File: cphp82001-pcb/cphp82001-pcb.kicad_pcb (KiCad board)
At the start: 2 copper layers, 56 x 44 mm, 32 parts, among them J1 USB_B_Micro, J2 PAD+, J3 PAD-, Q1 2N7002, U1 BQ21040, U2 TLV75801, U3 MAX40203AUK, U6 NCP360SNT

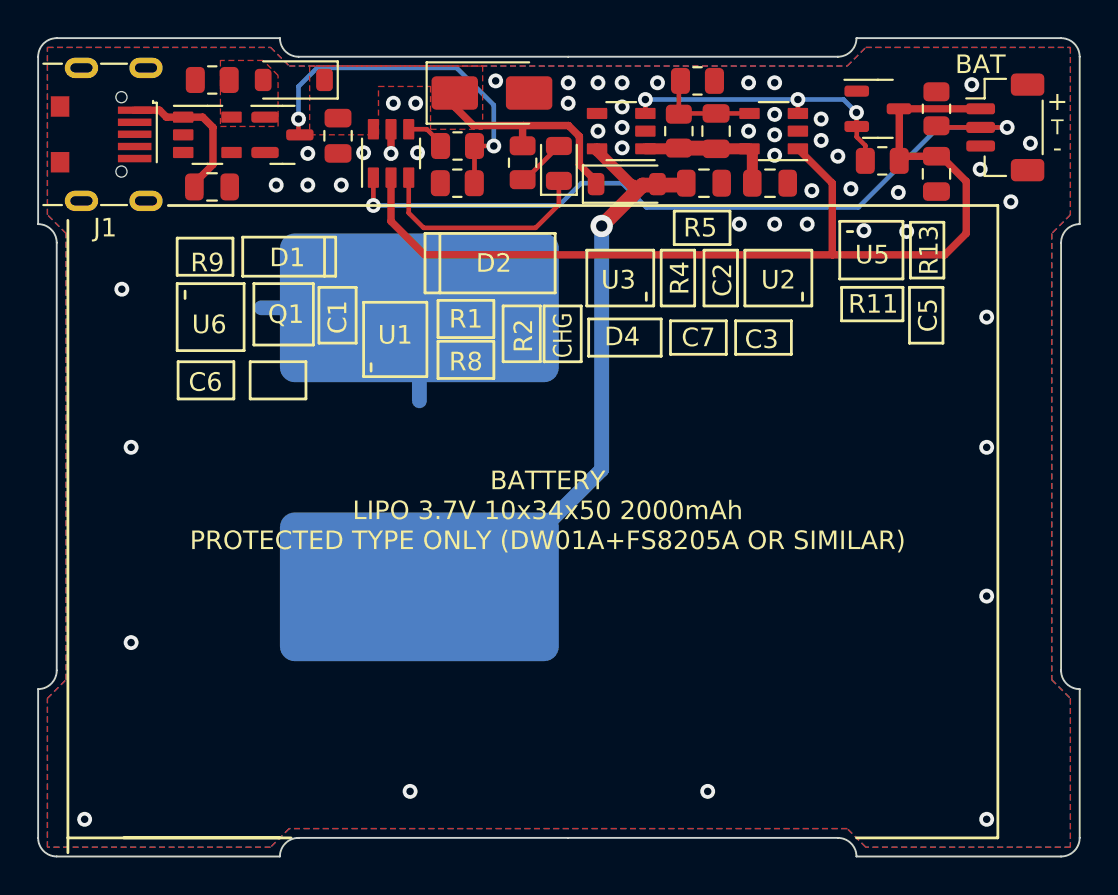
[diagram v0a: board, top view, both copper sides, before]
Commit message: rev3.3
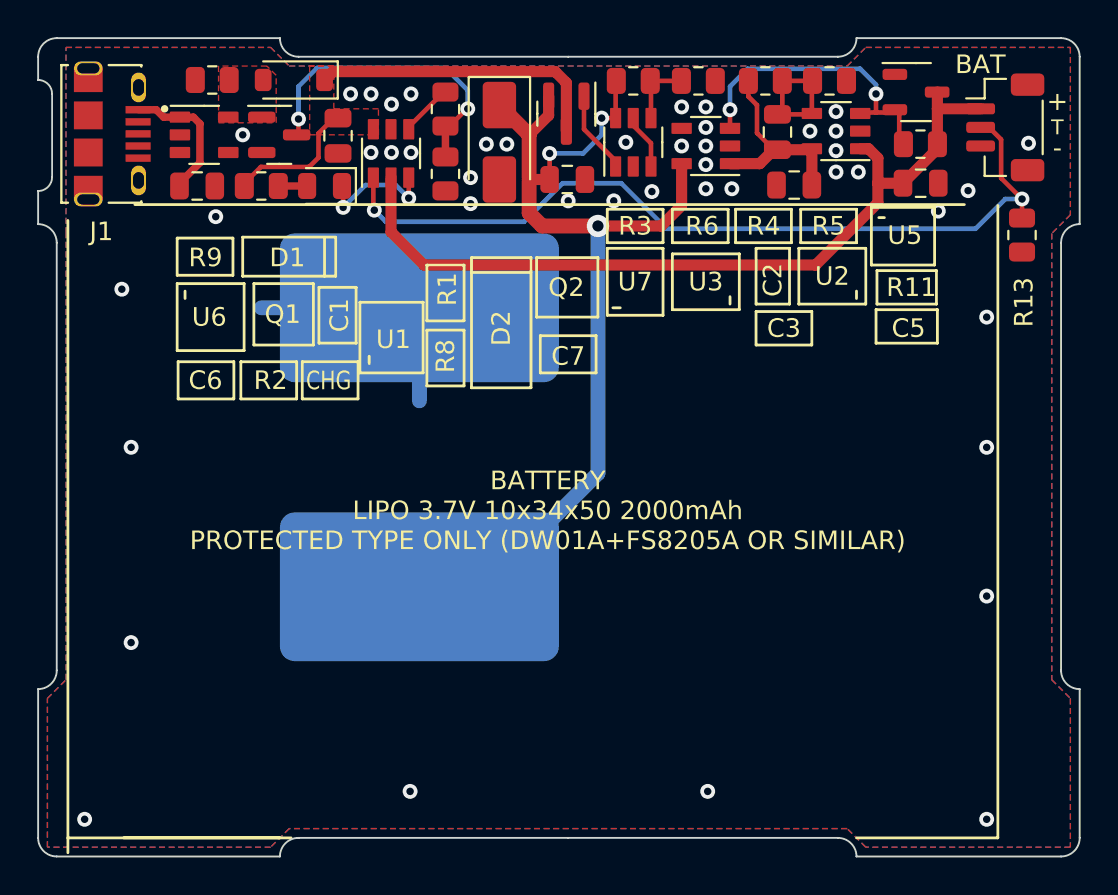
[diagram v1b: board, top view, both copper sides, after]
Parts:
- removed D4: PMEG40T10ERX, Diode_SMD:D_SOD-123
- added Q2: AO3401A, Package_TO_SOT_SMD:SOT-23, F.Cu at (28.4, 4.06)
- added R3: 560k, Resistor_SMD:R_0805_2012Metric, F.Cu at (32.0, 2.30)
- added R6: 220k, Resistor_SMD:R_0805_2012Metric, F.Cu at (35.5, 2.30)
- added U7: MCP65R41T-120E/CHY, george:SOT-23-6_TI_DBV6, F.Cu at (32.0, 5.60)
- J1: value USB_B_Micro -> USB; footprint george:USB_ALIEX_4LEG -> mod_local:AMPHENOL_10118194-0001LF
- U5: value ~ -> APX803S-SA
- moved R2 14.1 mm to (12.0, 7.95), turned to 180 degrees
- moved D3 12.7 mm to (15.4, 7.95), turned to 180 degrees
- moved R13 8.20 mm to (52.9, 10.6), turned to 90 degrees
- moved C7 7.35 mm to (28.4, 7.60)
- moved R5 7.10 mm to (42.5, 2.30)
- moved R4 5.38 mm to (39.1, 2.30), turned to 0 degrees
- moved U3 4.62 mm to (35.9, 5.80)
- moved U2 3.35 mm to (42.9, 5.00)
- moved C2 3.30 mm to (39.8, 5.05)
- moved D2 2.68 mm to (24.8, 5.60), turned to -90 degrees
- moved J1 2.52 mm to (2.70, 5.15)
- moved U5 2.24 mm to (47.2, 2.90)
- moved R11 2.24 mm to (47.4, 5.70)
- moved R1 2.09 mm to (21.9, 3.81), turned to 90 degrees
- moved C3 1.30 mm to (40.6, 7.90), turned to 180 degrees
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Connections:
- D2 pad 1: /VCC -> /VOUT
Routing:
- net /VOUT: track 30.7 -> 51.3 mm, vias 1 -> 3
- net /VCC: track 12.0 -> 23.1 mm
- net /B+: track 54.6 -> 43.9 mm
- net /CHG: track 11.9 -> 6.50 mm, vias 0 -> 2
- net /PASSG: track 0.00 -> 4.48 mm
- net /VCOMP: track 0.00 -> 3.64 mm
- net /VREG: track 7.44 -> 10.7 mm
- net /TS: track 41.9 -> 45.0 mm
- net /PROG2: track 19.6 -> 16.9 mm
- net Net-(U7-+): track 0.00 -> 2.59 mm
- net /ADJ: track 5.46 -> 6.78 mm
- net /GND: track 14.5 -> 13.5 mm, vias 50 -> 44
- net /LCHG: track 2.56 -> 1.55 mm
- net /PROG: track 2.02 -> 2.75 mm
- net /VBUS1: track 8.01 -> 7.29 mm
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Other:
- outline, holes or cut-outs redrawn

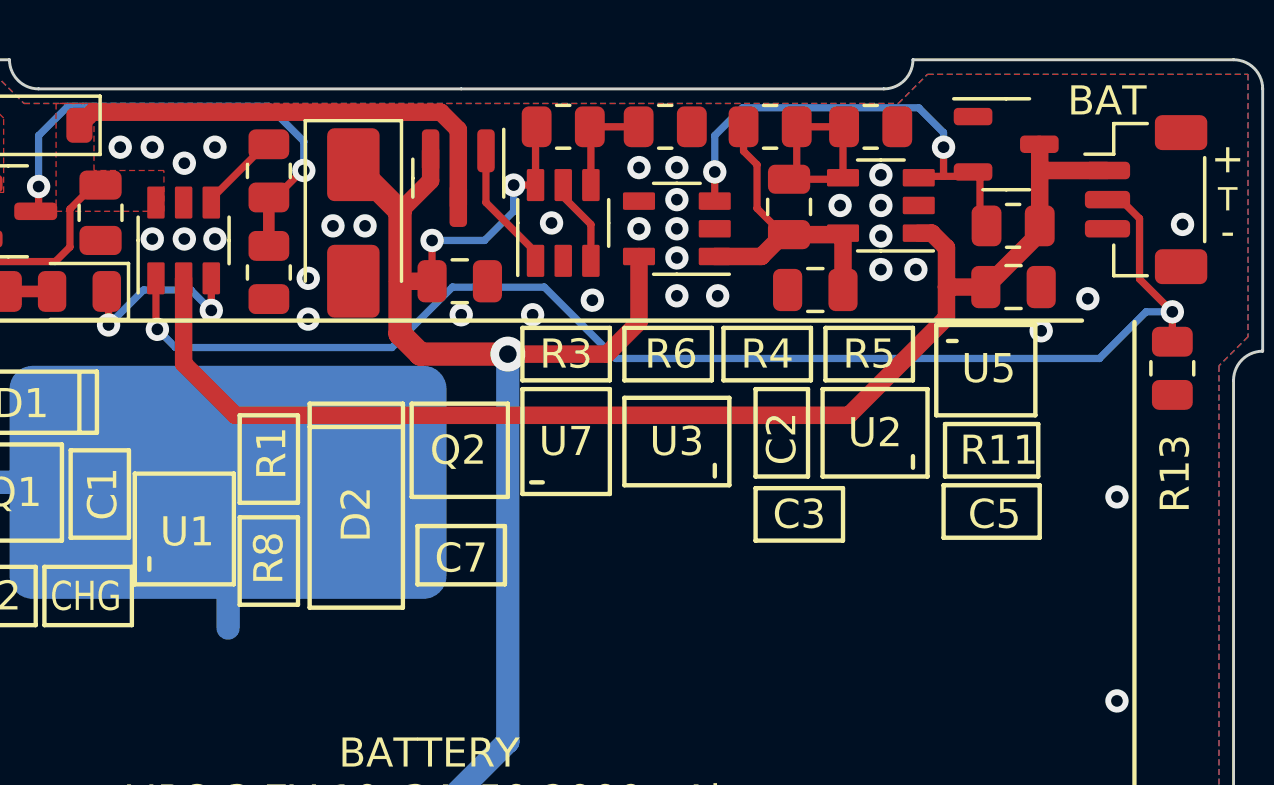
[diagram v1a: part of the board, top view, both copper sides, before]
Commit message: rev3.3a
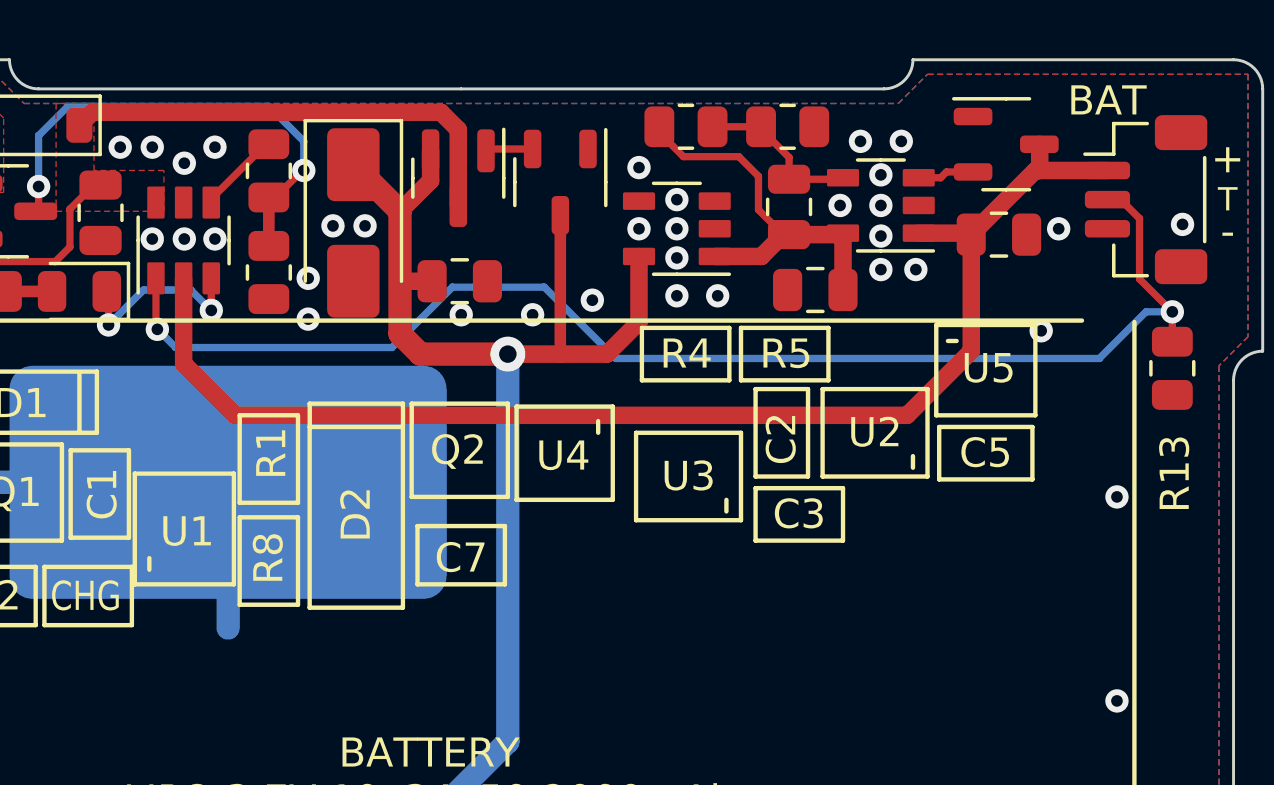
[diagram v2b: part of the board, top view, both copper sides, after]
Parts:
- removed R11: 1M, Resistor_SMD:R_0805_2012Metric
- removed R3: 560k, Resistor_SMD:R_0805_2012Metric
- removed R6: 220k, Resistor_SMD:R_0805_2012Metric
- removed U7: MCP65R41T-120E/CHY, george:SOT-23-6_TI_DBV6
- added U4: APX810-44SA, Package_TO_SOT_SMD:SOT-23-3, F.Cu at (31.9, 4.20)
- Q2: value AO3401A -> AO3413
- U5: value APX803S-SA -> APX809S-31SA
- moved R4 2.89 mm to (36.2, 2.30)
- moved R5 2.85 mm to (39.7, 2.30)
- moved C5 1.87 mm to (47.0, 6.00)
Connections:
- U3 pad 3: /EN -> unconnected-(U3-EN-Pad3)
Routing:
- net /EN: track 15.7 -> 1.95 mm, vias 2 -> 0
- net /VCOMP: track 3.64 -> 0.00 mm
- net /VOUT: track 51.3 -> 47.8 mm, vias 3 -> 1
- net /PASSG: track 4.48 -> 1.63 mm
- net Net-(U7-+): track 2.59 -> 0.00 mm
- net /VREG: track 10.7 -> 13.0 mm
- net /ADJ: track 6.78 -> 5.71 mm
